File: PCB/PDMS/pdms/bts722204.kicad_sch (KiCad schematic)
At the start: 22 parts, among them IC7 BTS722204ESAXUMA1

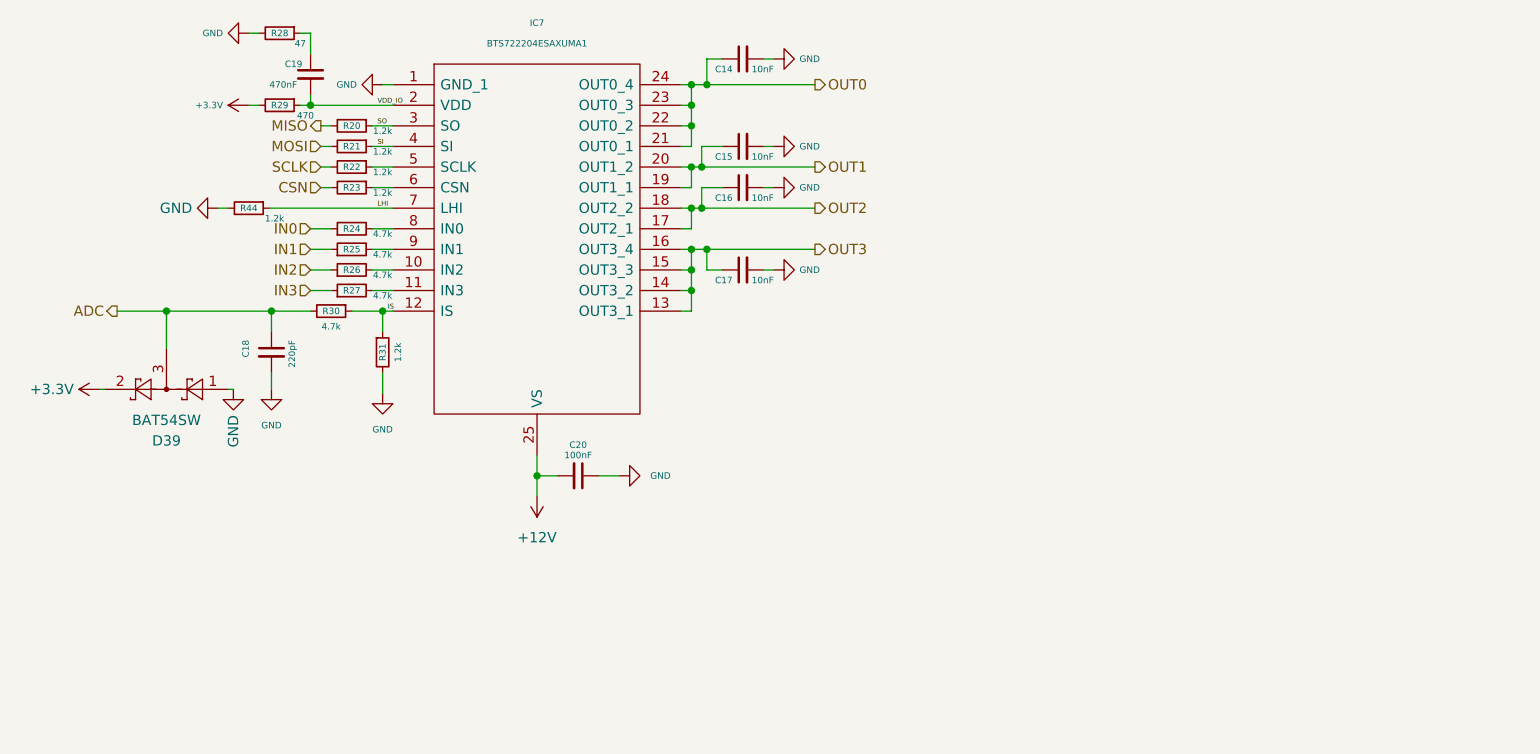
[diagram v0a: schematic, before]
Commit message: Finished 2024 version + gerbers
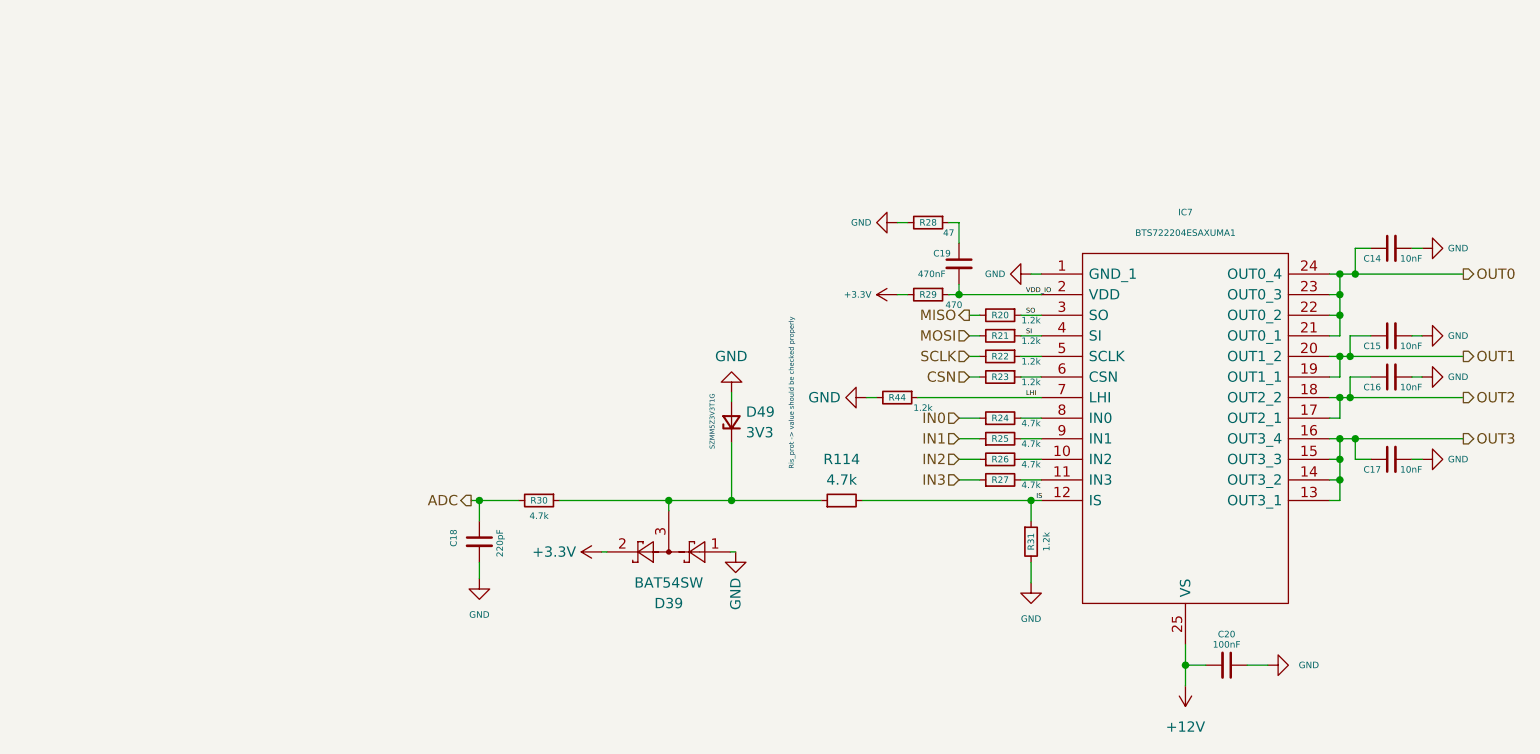
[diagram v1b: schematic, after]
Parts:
- added D49: 3V3, Diode_SMD:D_SOD-523, symbol Device:D_Zener_Small
- added R114: 4.7k, Resistor_SMD:R_0402_1005Metric, symbol Device:R_Small
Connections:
- net ADC: no longer D39.3
- net GND: now also D49.2 (A)
- net IS: now also R114.2; no longer R30.1
- new net: D39.3, D49.1 (K), R114.1, R30.1
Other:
- note added: "Ris_prot -> value should be checked properly"
- note added: "SZMM5Z3V3T1G"
- moved on the sheet: C14, C15, C16, C17, C18, C19, C20, D39, IC7, R20, R21, R22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
